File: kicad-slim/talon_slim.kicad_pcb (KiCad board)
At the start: 2 copper layers, 41 parts, among them J1 JST connector, SW1 SW_Push, SW10 SW_Push, SW11 SW_Push, SW12 SW_Push, SW13 SW_Push, SW14 SW_Push, SW15 SW_Push, SW16 SW_Push, SW17 SW_Push, SW18 SW_Push, SW19 SW_Push, SW2 SW_Push, SW20 SW_Push, SW3 SW_Push, SW4 SW_Push, SW5 SW_Push, SW6 SW_Push, SW7 SW_Push, SW8 SW_Push, SW9 SW_Push, U1 nice_nano

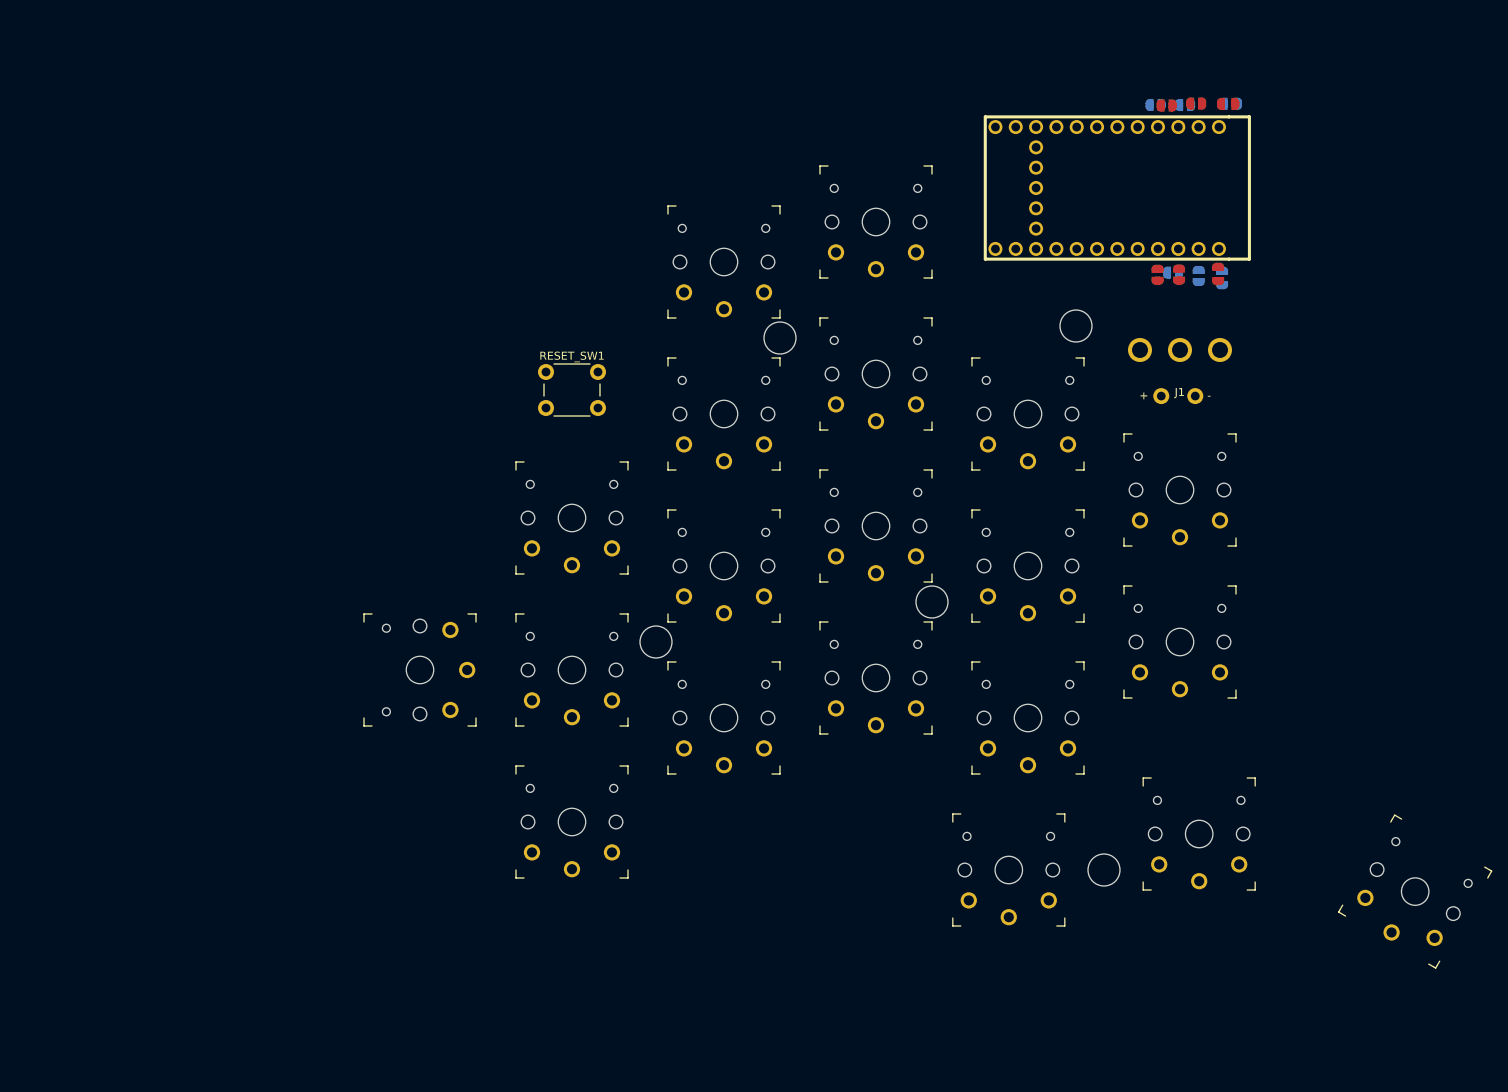
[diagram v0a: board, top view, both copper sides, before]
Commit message: Slim looking not tooooo bad
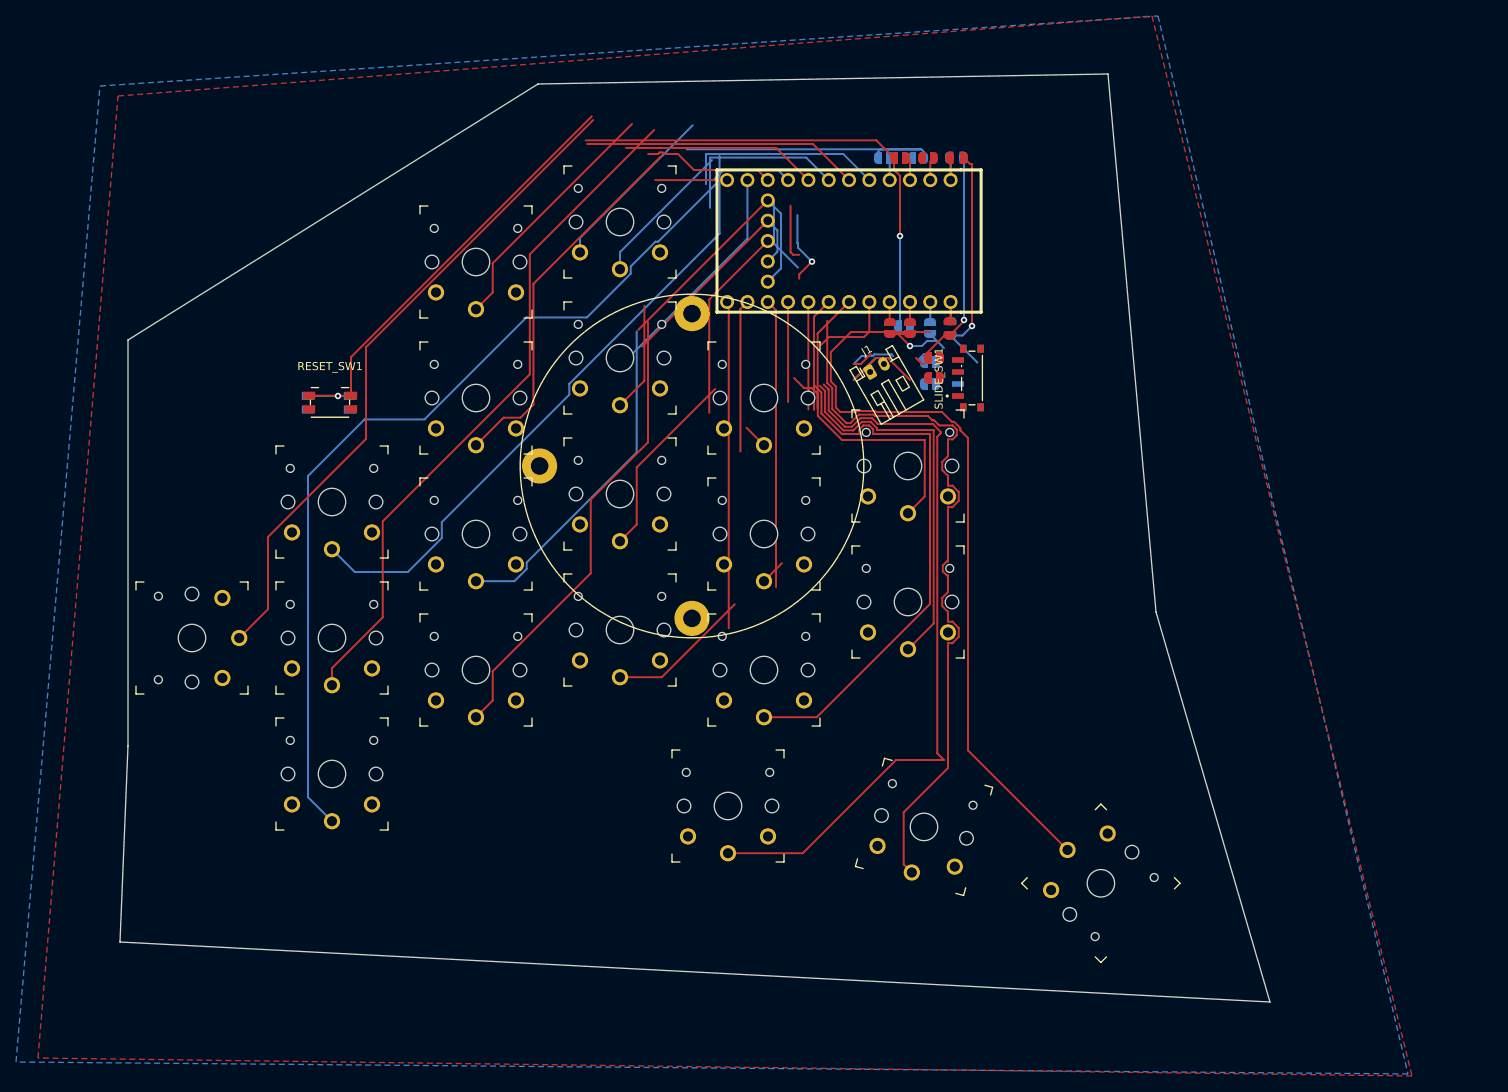
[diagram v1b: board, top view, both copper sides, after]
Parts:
- removed HOLE1, HOLE2, HOLE3, HOLE4: through_hole_m2, footprints:through_hole_m2
- removed the REF** at (157.0, 108.5)
- added JP10: Jumper_2_Open, footprints:Jumper_Open_0.5mm, F.Cu at (157.2, 78.0)
- added JP15: Jumper_2_Open, footprints:Jumper_Open_0.5mm, B.Cu at (156.8, 78.5)
- added JP16: Jumper_2_Open, footprints:Jumper_Open_0.5mm, F.Cu at (157.2, 80.5)
- added JP3: Jumper_2_Open, footprints:Jumper_Open_0.5mm, B.Cu at (156.8, 81.2)
- added REF**: Tenting Puck, footprints:SplitkbTentingPuck, F.Cu at (127.0, 91.5)
- added RESET_SW2: SW_Push, footprints:Panasonic_EVQPUL_EVQPUC, B.Cu at (81.6, 83.6)
- added SLIDE_SW2: SW_SPDT, footprints:SW_SSSS811101, B.Cu at (162.0, 80.5)
- J1: footprint footprints:power_connector -> Connector_JST:JST_PH_S2B-PH-K_1x02_P2.00mm_Horizontal
- RESET_SW1: footprint Button_Switch_THT:SW_PUSH_6mm -> footprints:Panasonic_EVQPUL_EVQPUC
- SLIDE_SW1: footprint footprints:slide_switch_5mm -> footprints:SW_SSSS811101
- SW18, SW20: footprint footprints:SW_PG1350_reversible -> footprints:SW_PG1350_reversible_1.5U
- moved SW20 39.3 mm to (178.1, 143.7), turned to -135 degrees
- moved J1 38.8 mm to (149.3, 79.8), turned to 30 degrees
- moved SW18 36.0 mm to (131.5, 134.0)
- moved JP2 35.0 mm to (159.8, 53.0)
- moved JP1 34.6 mm to (159.8, 53.0)
- moved JP7 34.6 mm to (151.0, 53.0)
- moved JP8 34.5 mm to (159.2, 74.0)
- moved SW19 34.4 mm to (156.0, 136.6), turned to -15 degrees
- moved SW13 34.4 mm to (154.0, 108.5)
- moved JP13 34.3 mm to (154.2, 74.2)
- moved JP12 34.3 mm to (153.5, 74.0)
- moved JP9 34.2 mm to (159.2, 74.0)
- moved JP11 34.2 mm to (156.8, 74.2)
- moved JP4 34.2 mm to (156.5, 53.0)
- moved U1 34.2 mm to (145.4, 63.4)
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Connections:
- J1 pad 2: GND -> Net-(J1-Pin_2)
- SLIDE_SW1 pad 2: Net-(J1-Pin_1) -> Net-(JP10-B)
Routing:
- net P7: track 0.00 -> 133.3 mm
- net P1: track 0.00 -> 122.9 mm, vias 0 -> 1
- net RESET: track 0.00 -> 118.8 mm, vias 0 -> 2
- net P6: track 0.00 -> 117.7 mm
- net P19: track 0.00 -> 107.8 mm
- net P20: track 0.00 -> 103.5 mm
- net P10: track 0.00 -> 102.5 mm
- net P9: track 0.00 -> 89.2 mm
- net P32: track 0.00 -> 86.6 mm
- net P17: track 0.00 -> 81.3 mm
- net GND: track 0.00 -> 70.3 mm, vias 0 -> 1
- net P11: track 0.00 -> 70.3 mm
- net P18: track 0.00 -> 62.0 mm
- net P13: track 0.00 -> 59.0 mm
- net P12: track 0.00 -> 56.0 mm
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- added copper zone on B.Cu, net GND
- added copper zone on F.Cu, net GND
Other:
- board outline added: 143.8 x 116 mm

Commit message: sent slim for procuction
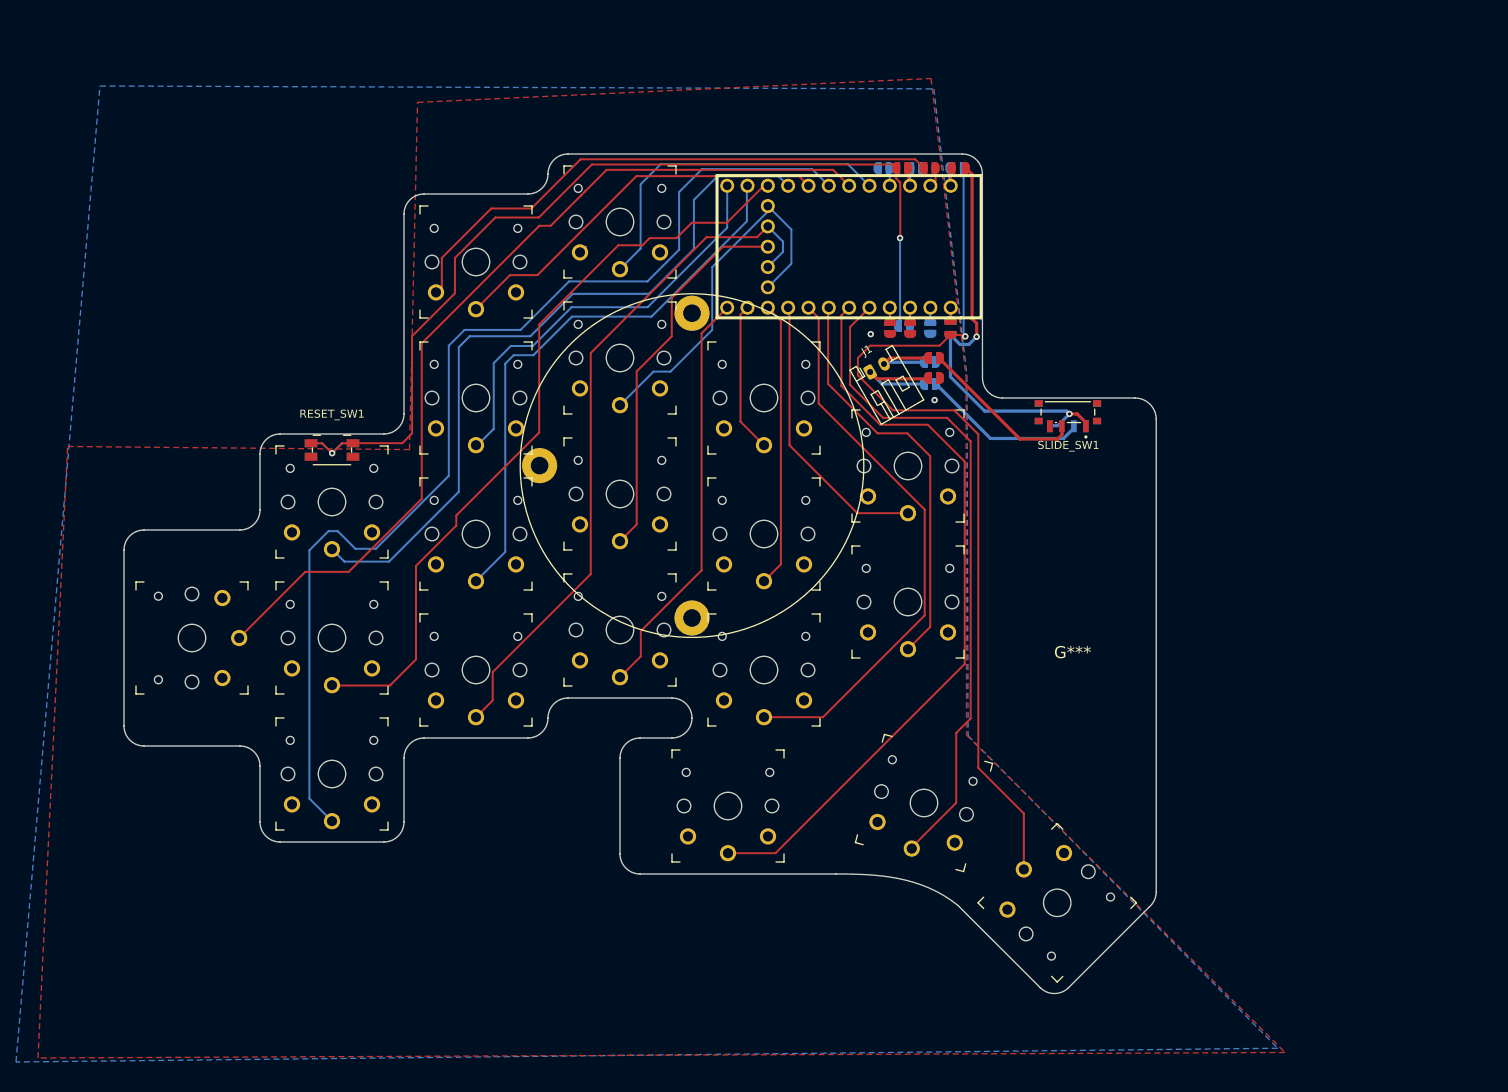
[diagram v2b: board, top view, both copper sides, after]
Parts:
- added G***: LOGO, footprints:handprint, F.Cu at (174.6, 114.8)
- SW20: footprint footprints:SW_PG1350_reversible_1.5U -> footprints:SW_PG1350_reversible
- SW8: footprint footprints:SW_PG1350_reversible -> footprints:SW_PG1350_reversible_1.5U
- moved SLIDE_SW2 12.7 mm to (174.0, 84.8), turned to 0 degrees
- moved SLIDE_SW1 12.7 mm to (174.0, 84.8), turned to 180 degrees
- moved SW20 5.98 mm to (172.7, 146.1)
- moved RESET_SW1 5.96 mm to (82.0, 89.5)
- moved RESET_SW2 5.91 mm to (82.0, 89.5)
- moved SW19 2.99 mm to (156.0, 133.6)
- moved JP2 1.30 mm to (159.8, 54.3)
- moved JP5 1.28 mm to (153.3, 54.2)
- moved JP1 1.28 mm to (160.0, 54.2)
- moved JP6 1.28 mm to (155.0, 54.3)
- moved JP4 1.26 mm to (156.7, 54.2)
- moved JP7 1.26 mm to (151.0, 54.3)
- moved U1 0.71 mm to (145.4, 64.1)
- moved JP9 0.12 mm to (159.3, 73.9)
- moved JP8 0.07 mm to (159.3, 73.9)
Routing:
- net P20: track 103.5 -> 82.6 mm
- net BATIN: track 38.9 -> 54.6 mm
- net P19: track 107.8 -> 94.2 mm
- net Net-(JP10-B): track 7.04 -> 20.6 mm
- net P17: track 81.3 -> 70.0 mm
- net Net-(JP3-B): track 9.74 -> 20.6 mm
- net P18: track 62.0 -> 51.4 mm
- net P1: track 122.9 -> 114.0 mm
- net P16: track 43.7 -> 35.6 mm
- net P13: track 59.0 -> 51.7 mm
- net P8: track 55.7 -> 48.9 mm
- net P10: track 102.5 -> 95.9 mm
- net RESET: track 118.8 -> 124.9 mm
- net P6: track 117.7 -> 112.7 mm
- net P15: track 39.3 -> 35.7 mm
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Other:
- board size 143.8 x 116 mm -> 129 x 104.9 mm
